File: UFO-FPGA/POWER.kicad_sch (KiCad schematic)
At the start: 24 parts

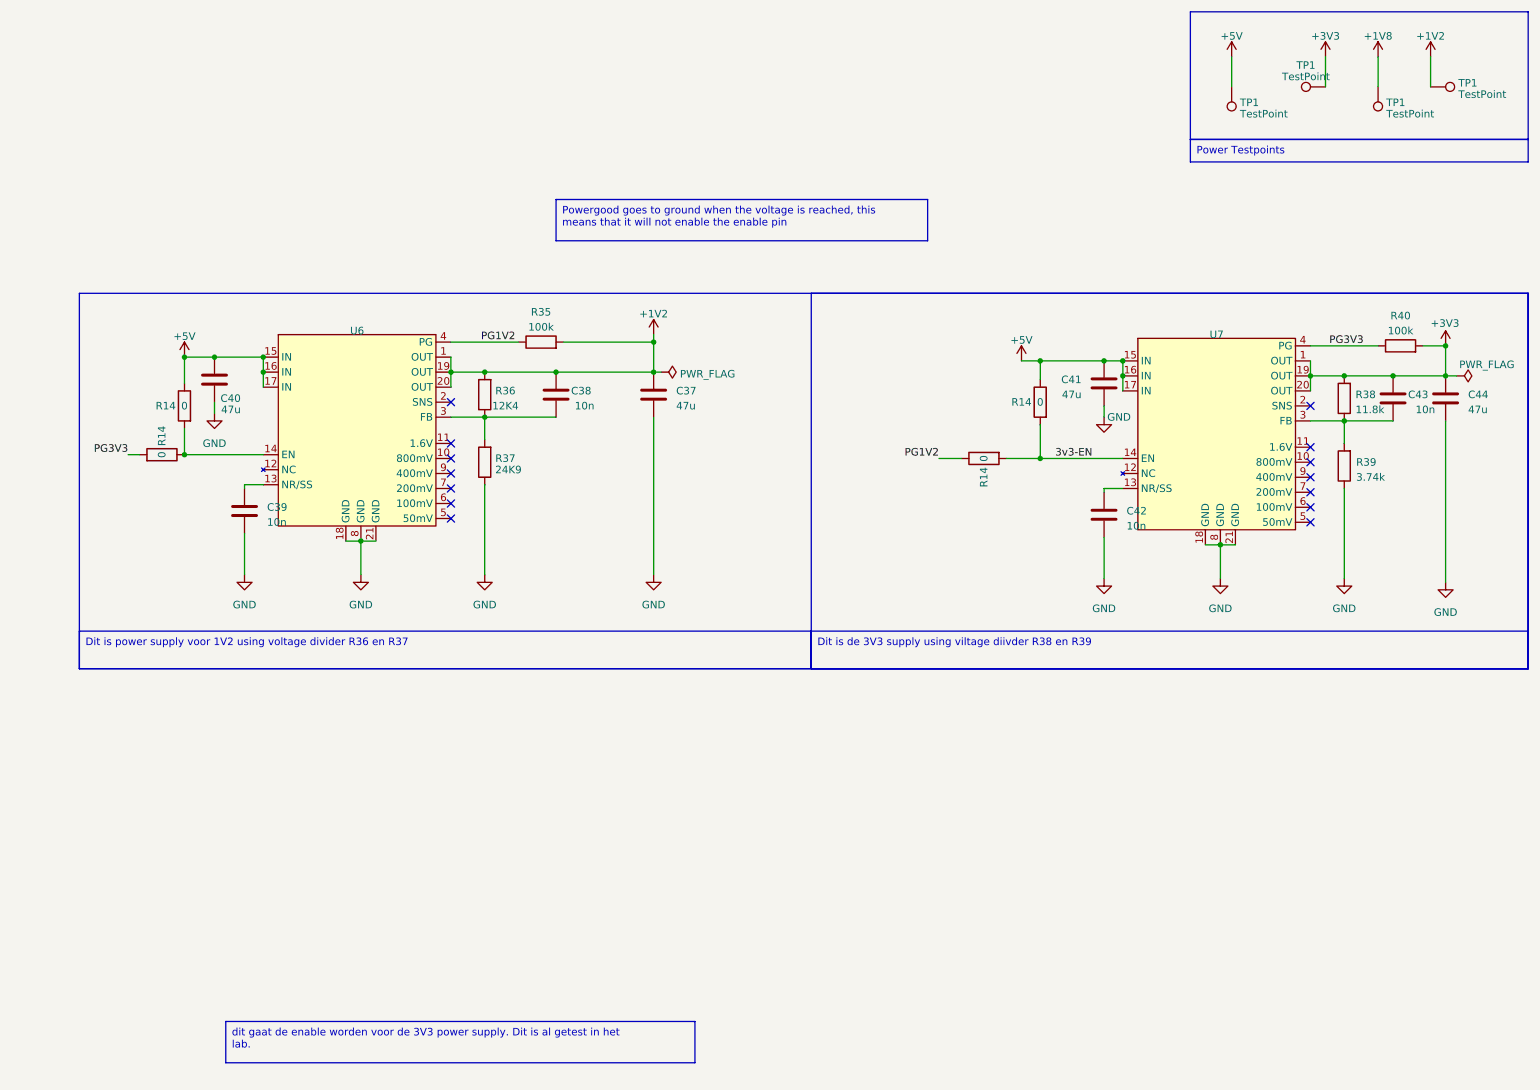
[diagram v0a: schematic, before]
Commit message: IO and power
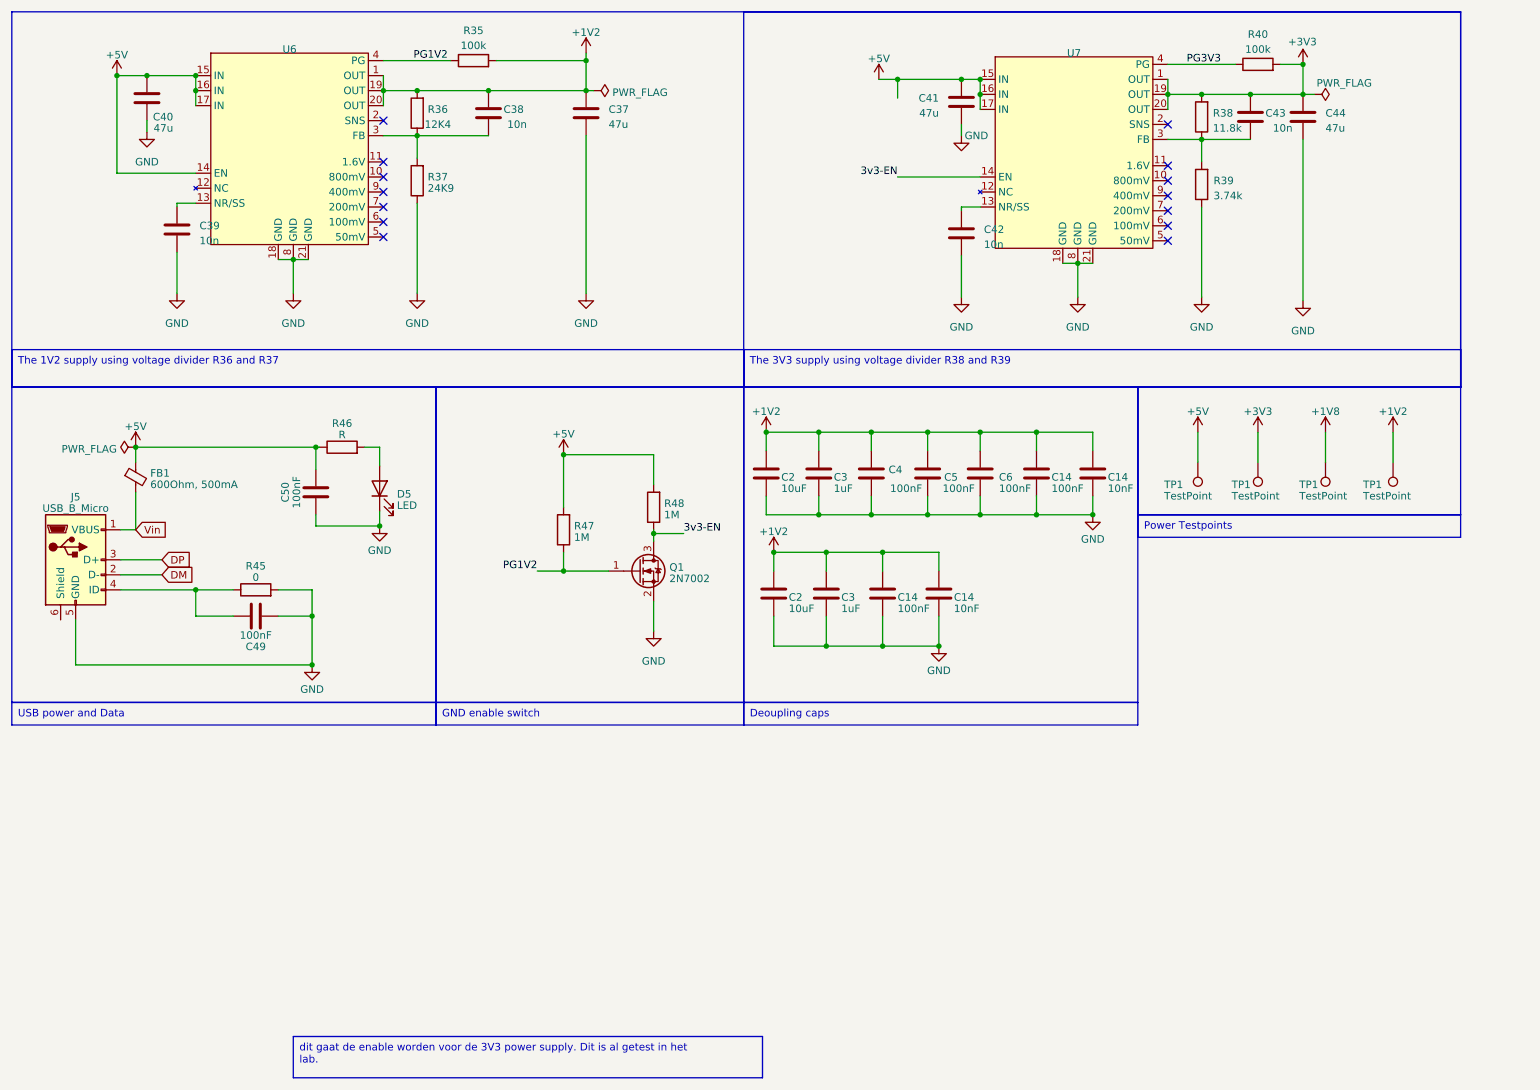
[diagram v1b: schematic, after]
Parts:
- removed R14 (x4): 0, symbol Device:R
- removed TP1 (x4): TestPoint, symbol Connector:TestPoint
- added C14 (x2): 10nF, symbol Device:C
- added C14 (x2), C4, C49, C5, C50, C6: 100nF, symbol Device:C
- added C2 (x2): 10uF, symbol Device:C
- added C3 (x2): 1uF, symbol Device:C
- added D5: LED, symbol Device:LED
- added FB1: 600Ohm, 500mA, symbol Device:FerriteBead_Small
- added J5: USB_B_Micro, symbol Connector:USB_B_Micro
- added Q1: 2N7002, Package_TO_SOT_SMD:SOT-23, symbol Transistor_FET:2N7002
- added R45: 0, symbol Device:R
- added R46: R, symbol Device:R
- added R47, R48: 1M, symbol Device:R
- added TP1 (x4): TestPoint, symbol Connector:TestPoint
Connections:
- net +1V2: now also C14.1, C14.1, C14.1, C14.1, C2.1, C2.1, C3.1, C3.1, C4.1, C5.1, C6.1, TP1.1
- net +1V8: now also TP1.1
- net +3V3: now also TP1.1
- net +5V: now also U6.14 (EN), C50.1, FB1.1, R46.1, R47.2, R48.2, TP1.1
- net 3v3-EN: now also Q1.3 (D), R48.1
- net GND: now also C14.2, C14.2, C14.2, C14.2, C2.2, C2.2, C3.2, C3.2, C4.2, C49.2, C5.2, C50.2, C6.2, D5.1 (K), J5.5 (GND), Q1.2 (S), R45.2
- net PG1V2: now also Q1.1 (G), R47.1
- new net: C49.1, J5.4 (ID), R45.1
- new net: D5.2 (A), R46.2
- new net DM: J5.2 (D-)
- new net DP: J5.3 (D+)
- new net Vin: FB1.2, J5.1 (VBUS)

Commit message: Revision
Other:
- company: (none) -> Universal-Field-Objects
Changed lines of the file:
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@@
   (title_block
     (title "UFO FPGA")
-    (date "2023-04-22")
-    (rev "V0.1")
+    (date "2023-04-25")
+    (rev "V0.5")
+    (company "Universal-Field-Objects")
   )
   (junction (at 161.925 106.68) (diameter 0) (color 0 0 0 0)
